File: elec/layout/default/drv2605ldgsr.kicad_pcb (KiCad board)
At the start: 2 copper layers, 225.7 x 100.8 mm, 3 parts

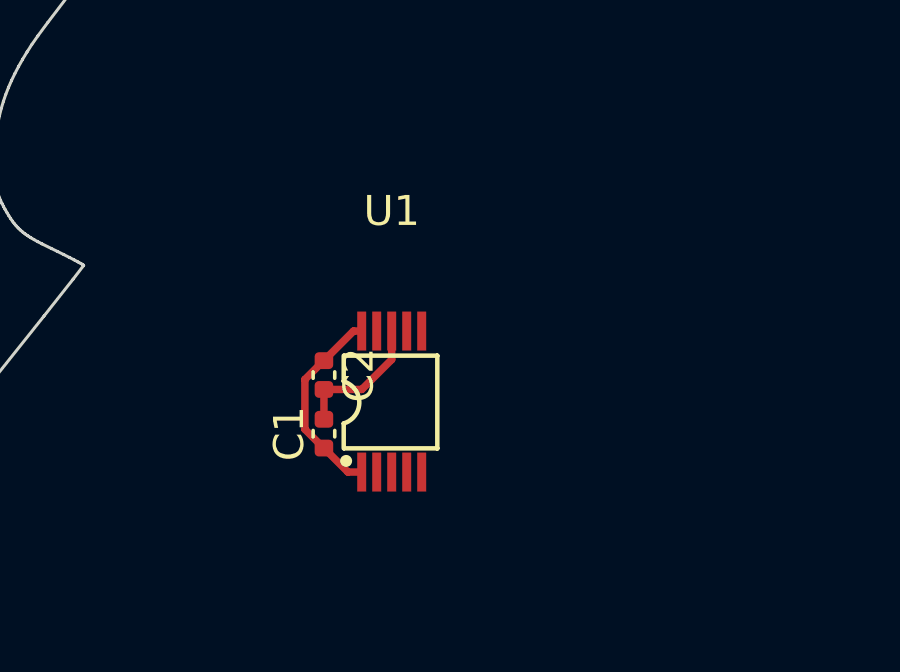
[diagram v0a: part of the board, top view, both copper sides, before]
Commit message: layout
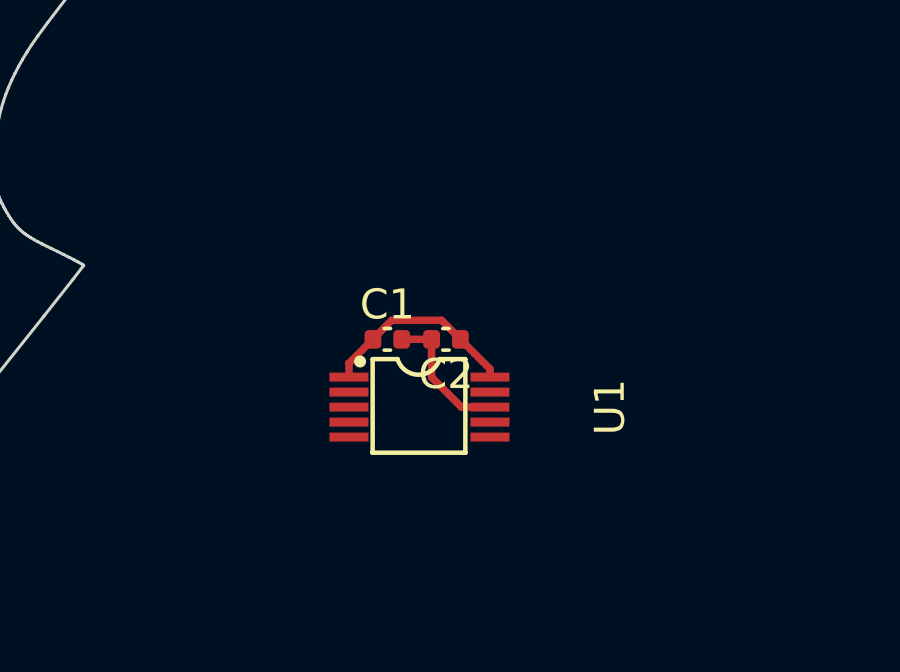
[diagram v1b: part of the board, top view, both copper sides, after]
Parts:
- moved C2 4.24 mm to (159.6, 90.5), turned to 180 degrees
- moved C1 3.79 mm to (157.7, 90.5), turned to 0 degrees
- moved U1 0.94 mm to (158.8, 92.7), turned to -90 degrees
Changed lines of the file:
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@@
   (net 9 "n")
   (footprint "lib:C0402" (layer "F.Cu")
-    (at 155.566181 91.641436 -90)
+    (at 159.633564 90.451181 180)
     (descr "Capacitor SMD 0402 (1005 Metric), square (rectangular) end terminal, IPC_7351 nominal, (Body size source: IPC-SM-782 page 76, https://www.pcb-3d.com/wordpress/wp-content/uploads/ipc-sm-782a_amendment_1_and_2.pdf), generated with kicad-footprint-generator")
     (tags "capacitor")
     (attr smd)
-    (fp_text reference "C2" (at 0 -1.16 90) (layer "F.SilkS")
+    (fp_text reference "C2" (at 0 -1.16) (layer "F.SilkS")
         (effects (font (size 1 1) (thickness 0.15)))
     )
-    (fp_text value "Multilayer Ceramic Capacitors MLCC - SMD/SMT 1uF 6.3V 0402 RoHS" (at 0 1.16 90) (layer "F.Fab")
+    (fp_text value "Multilayer Ceramic Capacitors MLCC - SMD/SMT 1uF 6.3V 0402 RoHS" (at 0 1.16) (layer "F.Fab")
         (effects (font (size 1 1) (thickness 0.15)))
     )
-    (fp_text user "${REFERENCE}" (at 0 0 90) (layer "F.Fab")
+    (fp_text user "${REFERENCE}" (at 0 0) (layer "F.Fab")
         (effects (font (size 0.25 0.25) (thickness 0.04)))
     )
@@
     (fp_line (start 0.5 0.25) (end -0.5 0.25)
       (stroke (width 0.1) (type solid)) (layer "F.Fab"))
-    (pad "1" smd roundrect (at -0.48 0 270) (size 0.56 0.62) (layers "F.Cu" "F.Paste" "F.Mask") (roundrect_rratio 0.25)
+    (pad "1" smd roundrect (at -0.48 0 180) (size 0.56 0.62) (layers "F.Cu" "F.Paste" "F.Mask") (roundrect_rratio 0.25)
       (net 1 "vcc") (pintype "stereo"))
-    (pad "2" smd roundrect (at 0.48 0 270) (size 0.56 0.62) (layers "F.Cu" "F.Paste" "F.Mask") (roundrect_rratio 0.25)
+    (pad "2" smd roundrect (at 0.48 0 180) (size 0.56 0.62) (layers "F.Cu" "F.Paste" "F.Mask") (roundrect_rratio 0.25)
       (net 8 "gnd") (pintype "stereo"))
     (model "${KICAD6_3DMODEL_DIR}/Capacitor_SMD.3dshapes/C_0402_1005Metric.wrl"
@@
   )
   (footprint "lib:VSSOP-10_L3.0-W3.0-P0.50-LS4.9-BL" (layer "F.Cu")
-    (at 157.825 92.525)
+    (at 158.75 92.71 -90)
     (attr smd)
-    (fp_text reference "U1" (at 0 -6.35) (layer "F.SilkS")
+    (fp_text reference "U1" (at 0 -6.35 90) (layer "F.SilkS")
         (effects (font (size 1 1) (thickness 0.15)))
     )
-    (fp_text value "" (at 0 6.35) (layer "F.Fab")
+    (fp_text value "" (at 0 6.35 90) (layer "F.Fab")
         (effects (font (size 1 1) (thickness 0.15)))
     )
-    (fp_text user "${REFERENCE}" (at 0 0) (layer "F.Fab")
+    (fp_text user "${REFERENCE}" (at 0 0 90) (layer "F.Fab")
         (effects (font (size 1 1) (thickness 0.15)))
     )
@@
     (fp_circle (center -1.5 2.45) (end -1.47 2.45)
       (stroke (width 0.06) (type solid)) (fill none) (layer "F.Fab"))
-    (pad "1" smd rect (at -1 2.35) (size 0.3 1.3) (layers "F.Cu" "F.Paste" "F.Mask")
+    (pad "1" smd rect (at -1 2.35 270) (size 0.3 1.3) (layers "F.Cu" "F.Paste" "F.Mask")
       (net 1 "vcc") (pintype "stereo"))
-    (pad "2" smd rect (at -0.5 2.35) (size 0.3 1.3) (layers "F.Cu" "F.Paste" "F.Mask")
+    (pad "2" smd rect (at -0.5 2.35 270) (size 0.3 1.3) (layers "F.Cu" "F.Paste" "F.Mask")
       (net 2 "scl") (pintype "stereo"))
-    (pad "3" smd rect (at 0 2.35) (size 0.3 1.3) (layers "F.Cu" "F.Paste" "F.Mask")
+    (pad "3" smd rect (at 0 2.35 270) (size 0.3 1.3) (layers "F.Cu" "F.Paste" "F.Mask")
       (net 3 "sda") (pintype "stereo"))
-    (pad "4" smd rect (at 0.5 2.35) (size 0.3 1.3) (layers "F.Cu" "F.Paste" "F.Mask")
+    (pad "4" smd rect (at 0.5 2.35 270) (size 0.3 1.3) (layers "F.Cu" "F.Paste" "F.Mask")
       (net 4 "in_trig") (pintype "stereo"))
-    (pad "5" smd rect (at 1 2.35) (size 0.3 1.3) (layers "F.Cu" "F.Paste" "F.Mask")
+    (pad "5" smd rect (at 1 2.35 270) (size 0.3 1.3) (layers "F.Cu" "F.Paste" "F.Mask")
       (net 5 "en") (pintype "stereo"))
-    (pad "6" smd rect (at 1 -2.35) (size 0.3 1.3) (layers "F.Cu" "F.Paste" "F.Mask")
+    (pad "6" smd rect (at 1 -2.35 270) (size 0.3 1.3) (layers "F.Cu" "F.Paste" "F.Mask")
       (net 6 "vdd_nc") (pintype "stereo"))
-    (pad "7" smd rect (at 0.5 -2.35) (size 0.3 1.3) (layers "F.Cu" "F.Paste" "F.Mask")
+    (pad "7" smd rect (at 0.5 -2.35 270) (size 0.3 1.3) (layers "F.Cu" "F.Paste" "F.Mask")
       (net 7 "p") (pintype "stereo"))
-    (pad "8" smd rect (at 0 -2.35) (size 0.3 1.3) (layers "F.Cu" "F.Paste" "F.Mask")
+    (pad "8" smd rect (at 0 -2.35 270) (size 0.3 1.3) (layers "F.Cu" "F.Paste" "F.Mask")
       (net 8 "gnd") (pintype "stereo"))
-    (pad "9" smd rect (at -0.5 -2.35) (size 0.3 1.3) (layers "F.Cu" "F.Paste" "F.Mask")
+    (pad "9" smd rect (at -0.5 -2.35 270) (size 0.3 1.3) (layers "F.Cu" "F.Paste" "F.Mask")
       (net 9 "n") (pintype "stereo"))
-    (pad "10" smd rect (at -1 -2.35) (size 0.3 1.3) (layers "F.Cu" "F.Paste" "F.Mask")
+    (pad "10" smd rect (at -1 -2.35 270) (size 0.3 1.3) (layers "F.Cu" "F.Paste" "F.Mask")
       (net 1 "vcc") (pintype "stereo"))
     (model "/Users/narayanpowderly/Documents/atopile-workspace/swoop/.ato/modules/drv2605ldgsr/elec/footprints/footprints.3dshapes/VSSOP-10_L3.0-W3.0-H1.1-LS4.9-P0.50.wrl"
@@
   )
   (footprint "lib:C0402" (layer "F.Cu")
-    (at 155.566181 93.595775 90)
+    (at 157.679225 90.451181)
     (descr "Capacitor SMD 0402 (1005 Metric), square (rectangular) end terminal, IPC_7351 nominal, (Body size source: IPC-SM-782 page 76, https://www.pcb-3d.com/wordpress/wp-content/uploads/ipc-sm-782a_amendment_1_and_2.pdf), generated with kicad-footprint-generator")
     (tags "capacitor")
     (attr smd)
-    (fp_text reference "C1" (at 0 -1.16 90) (layer "F.SilkS")
+    (fp_text reference "C1" (at 0 -1.16) (layer "F.SilkS")
         (effects (font (size 1 1) (thickness 0.15)))
     )
-    (fp_text value "Multilayer Ceramic Capacitors MLCC - SMD/SMT 1uF 6.3V 0402 RoHS" (at 0 1.16 90) (layer "F.Fab")
+    (fp_text value "Multilayer Ceramic Capacitors MLCC - SMD/SMT 1uF 6.3V 0402 RoHS" (at 0 1.16) (layer "F.Fab")
         (effects (font (size 1 1) (thickness 0.15)))
     )
-    (fp_text user "${REFERENCE}" (at 0 0 90) (layer "F.Fab")
+    (fp_text user "${REFERENCE}" (at 0 0) (layer "F.Fab")
         (effects (font (size 0.25 0.25) (thickness 0.04)))
     )
@@
     (fp_line (start 0.5 0.25) (end -0.5 0.25)
       (stroke (width 0.1) (type solid)) (layer "F.Fab"))
-    (pad "1" smd roundrect (at -0.48 0 90) (size 0.56 0.62) (layers "F.Cu" "F.Paste" "F.Mask") (roundrect_rratio 0.25)
+    (pad "1" smd roundrect (at -0.48 0) (size 0.56 0.62) (layers "F.Cu" "F.Paste" "F.Mask") (roundrect_rratio 0.25)
       (net 1 "vcc") (pintype "stereo"))
-    (pad "2" smd roundrect (at 0.48 0 90) (size 0.56 0.62) (layers "F.Cu" "F.Paste" "F.Mask") (roundrect_rratio 0.25)
+    (pad "2" smd roundrect (at 0.48 0) (size 0.56 0.62) (layers "F.Cu" "F.Paste" "F.Mask") (roundrect_rratio 0.25)
       (net 8 "gnd") (pintype "stereo"))
     (model "${KICAD6_3DMODEL_DIR}/Capacitor_SMD.3dshapes/C_0402_1005Metric.wrl"
@@
     (effects (font (size 2 2) (thickness 0.1)) (justify left bottom))
   )
-  (segment (start 156.365406 94.875) (end 155.566181 94.075775) (width 0.25) (layer "F.Cu") (net 1))
-  (segment (start 154.931181 93.448384) (end 155.558572 94.075775) (width 0.25) (layer "F.Cu") (net 1))
-  (segment (start 156.825 94.875) (end 156.365406 94.875) (width 0.25) (layer "F.Cu") (net 1))
-  (segment (start 156.825 90.175) (end 156.552617 90.175) (width 0.25) (layer "F.Cu") (net 1))
-  (segment (start 155.558572 91.161436) (end 154.931181 91.788827) (width 0.25) (layer "F.Cu") (net 1))
-  (segment (start 155.558572 94.075775) (end 155.566181 94.075775) (width 0.25) (layer "F.Cu") (net 1))
-  (segment (start 154.931181 91.788827) (end 154.931181 93.448384) (width 0.25) (layer "F.Cu") (net 1))
-  (segment (start 155.566181 91.161436) (end 155.558572 91.161436) (width 0.25) (layer "F.Cu") (net 1))
-  (segment (start 156.552617 90.175) (end 155.566181 91.161436) (width 0.25) (layer "F.Cu") (net 1))
-  (segment (start 157.825 90.175) (end 157.825 91.125) (width 0.25) (layer "F.Cu") (net 8))
-  (segment (start 155.566181 93.115775) (end 155.566181 92.121436) (width 0.25) (layer "F.Cu") (net 8))
-  (segment (start 157.825 91.125) (end 156.828564 92.121436) (width 0.25) (layer "F.Cu") (net 8))
-  (segment (start 156.828564 92.121436) (end 155.566181 92.121436) (width 0.25) (layer "F.Cu") (net 8))
+  (segment (start 156.4 91.250406) (end 157.199225 90.451181) (width 0.25) (layer "F.Cu") (net 1))
+  (segment (start 157.826616 89.816181) (end 157.199225 90.443572) (width 0.25) (layer "F.Cu") (net 1))
+  (segment (start 156.4 91.71) (end 156.4 91.250406) (width 0.25) (layer "F.Cu") (net 1))
+  (segment (start 161.1 91.71) (end 161.1 91.437617) (width 0.25) (layer "F.Cu") (net 1))
+  (segment (start 160.113564 90.443572) (end 159.486173 89.816181) (width 0.25) (layer "F.Cu") (net 1))
+  (segment (start 157.199225 90.443572) (end 157.199225 90.451181) (width 0.25) (layer "F.Cu") (net 1))
+  (segment (start 159.486173 89.816181) (end 157.826616 89.816181) (width 0.25) (layer "F.Cu") (net 1))
+  (segment (start 160.113564 90.451181) (end 160.113564 90.443572) (width 0.25) (layer "F.Cu") (net 1))
+  (segment (start 161.1 91.437617) (end 160.113564 90.451181) (width 0.25) (layer "F.Cu") (net 1))
+  (segment (start 161.1 92.71) (end 160.15 92.71) (width 0.25) (layer "F.Cu") (net 8))
+  (segment (start 158.159225 90.451181) (end 159.153564 90.451181) (width 0.25) (layer "F.Cu") (net 8))
+  (segment (start 160.15 92.71) (end 159.153564 91.713564) (width 0.25) (layer "F.Cu") (net 8))
+  (segment (start 159.153564 91.713564) (end 159.153564 90.451181) (width 0.25) (layer "F.Cu") (net 8))
   (group "" (id 6c1ef9f7-0f34-47bb-ac1a-76df23fb396e)
     (members
